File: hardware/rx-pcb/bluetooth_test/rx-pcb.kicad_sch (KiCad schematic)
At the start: 39 parts, among them J1 Conn_01x05_Pin, J2 Conn_01x04_Pin, J3 Conn_Coaxial_Small, J4 Conn_01x04_Pin, J6 Conn_01x03_Pin, SW1 SW_SPST, U1 STM32WB05KZV6TR, U2 STS4L-AD1B-R3, U3 STS4L-AD1B-R3, X1 Q22FA12800025, X2 ABS07-32.768KHZ-1-T

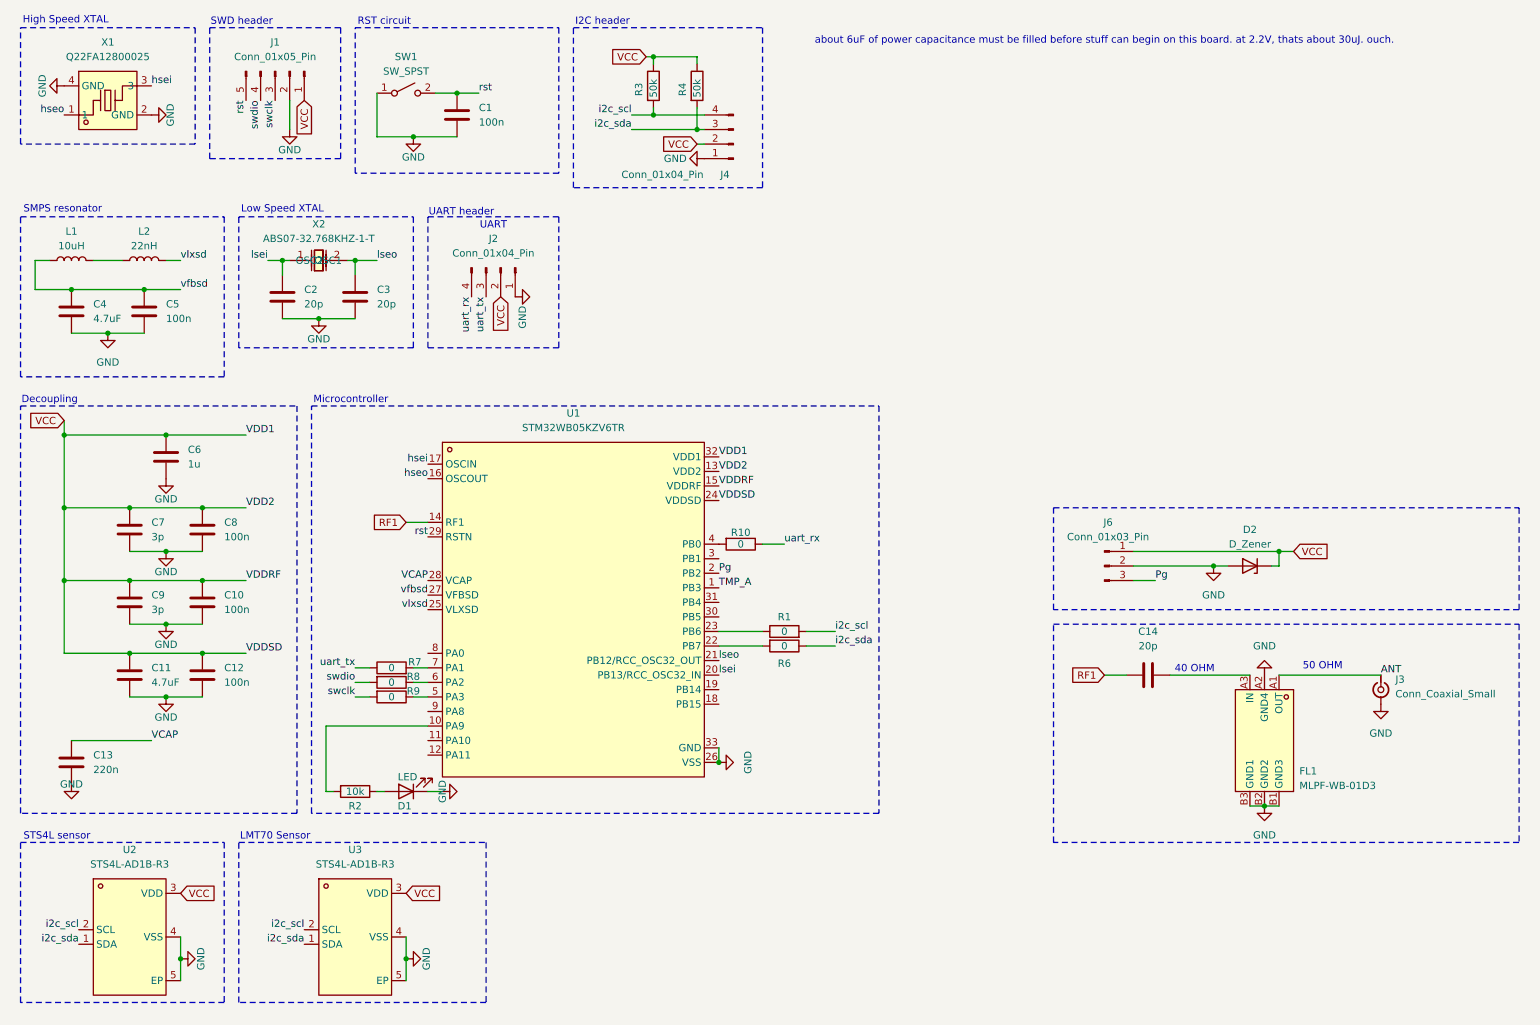
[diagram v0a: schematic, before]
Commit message: adapter + tx updates
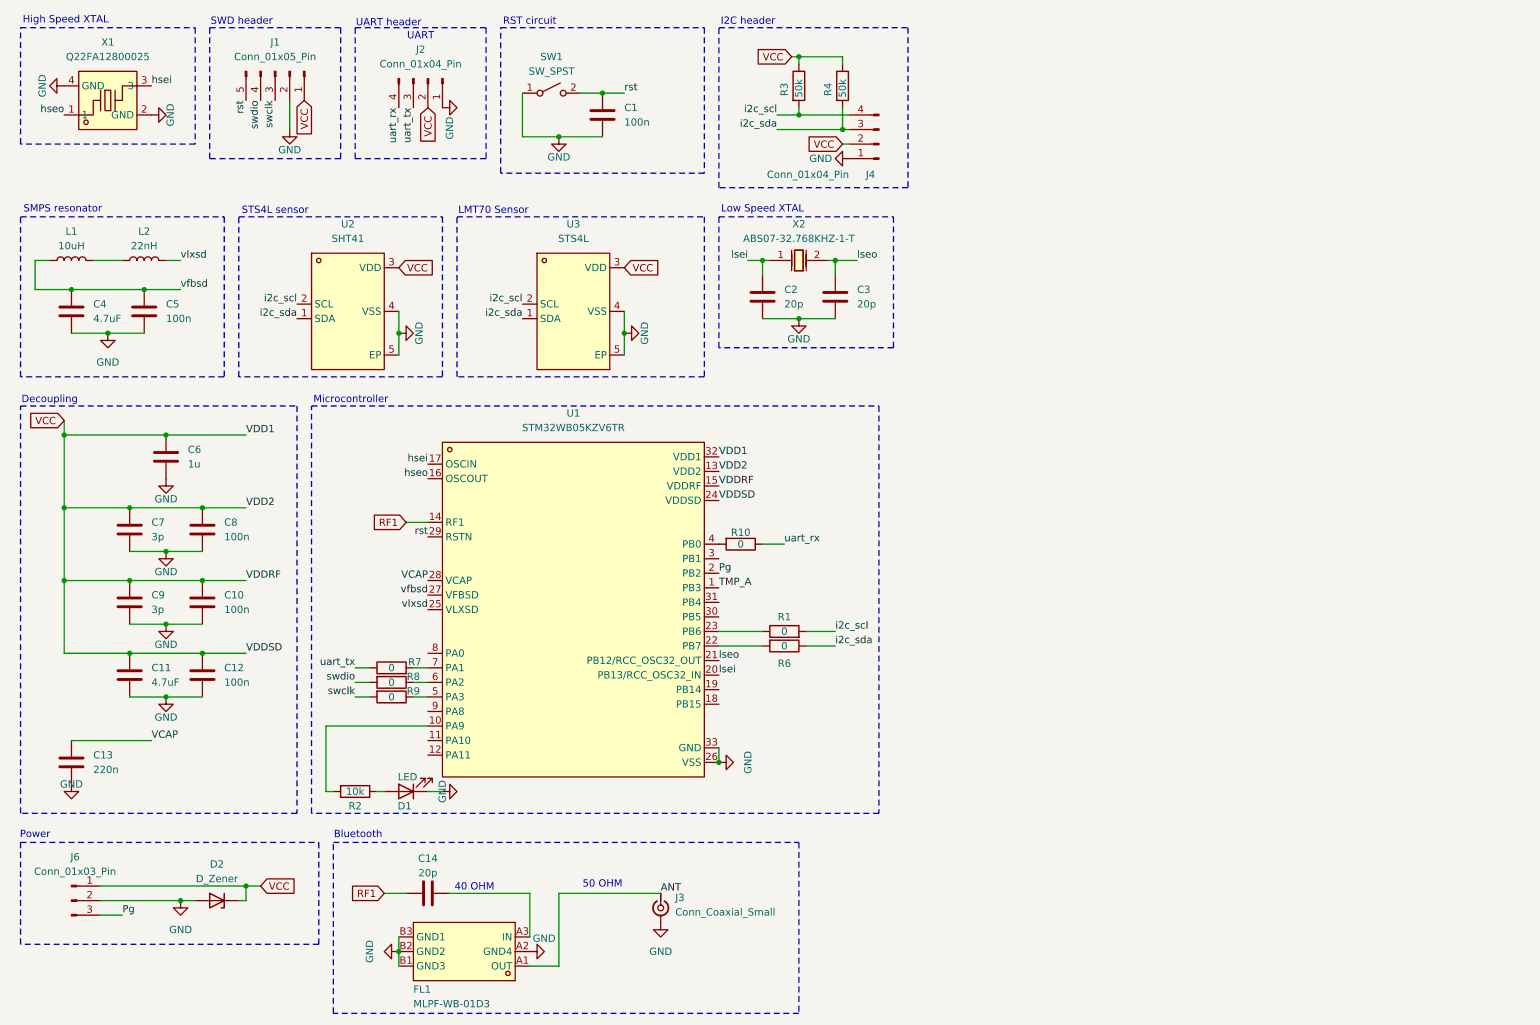
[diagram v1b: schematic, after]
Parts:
- U2: value STS4L-AD1B-R3 -> SHT41
- U3: value STS4L-AD1B-R3 -> STS4L
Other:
- note added: "Bluetooth"
- note added: "Power"
- note removed: "about 6uF of power capacitance must be filled before stuff can begin on this board. at 2.2V, thats about 30uJ. ouch."
- moved on the sheet: C1, C14, C2, C3, D2, FL1, J2, J3, J4, J6, R3, R4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
